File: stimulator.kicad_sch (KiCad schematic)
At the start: 1 part, among them U1 ENS001-A2

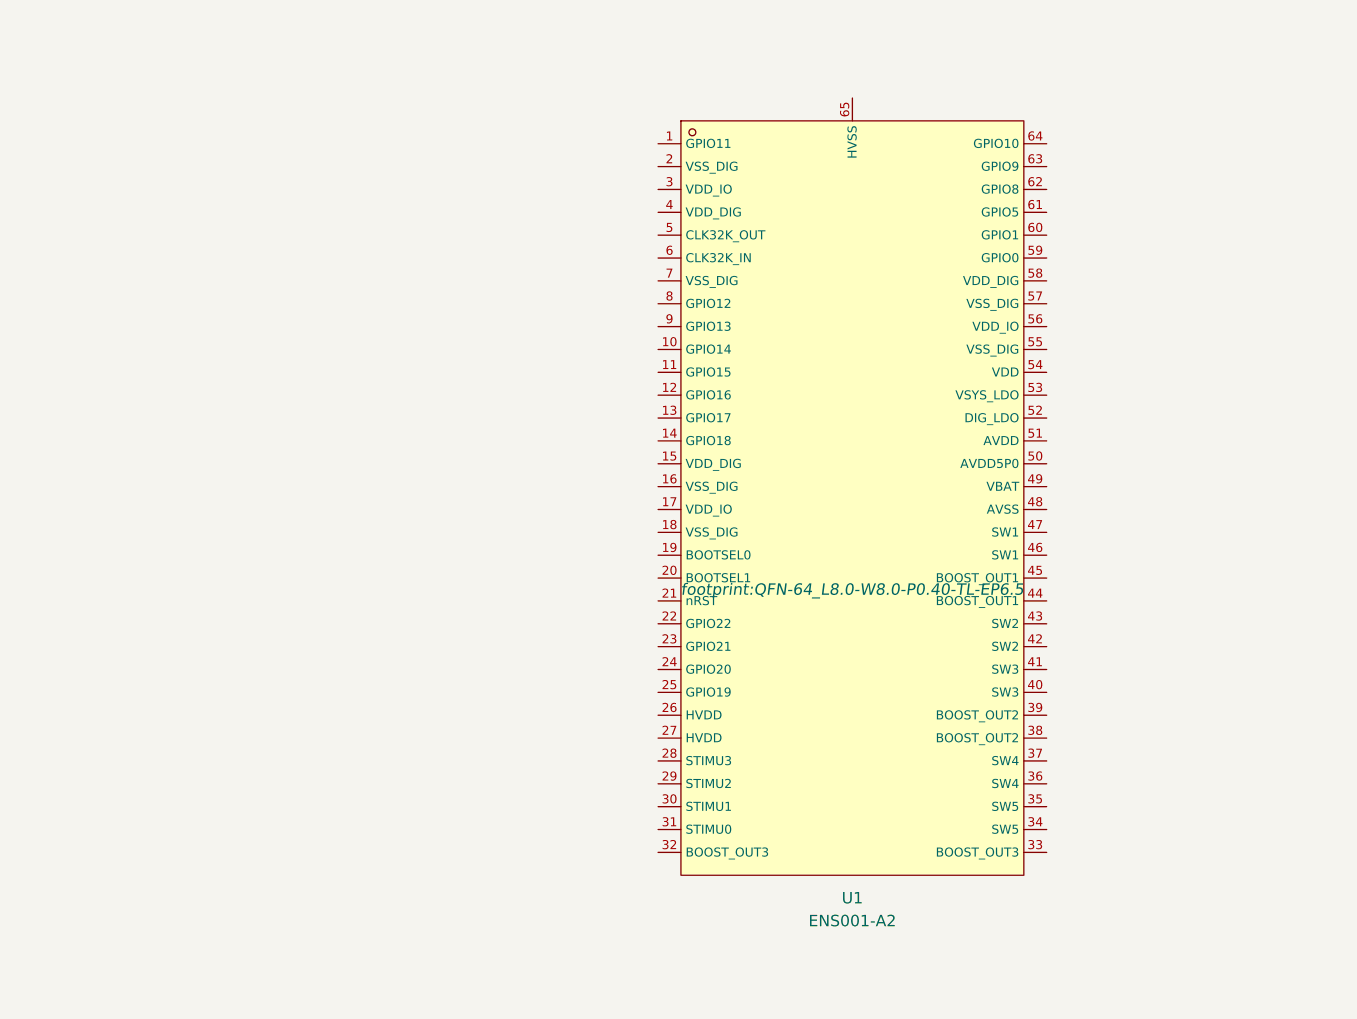
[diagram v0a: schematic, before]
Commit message: pin names assigned
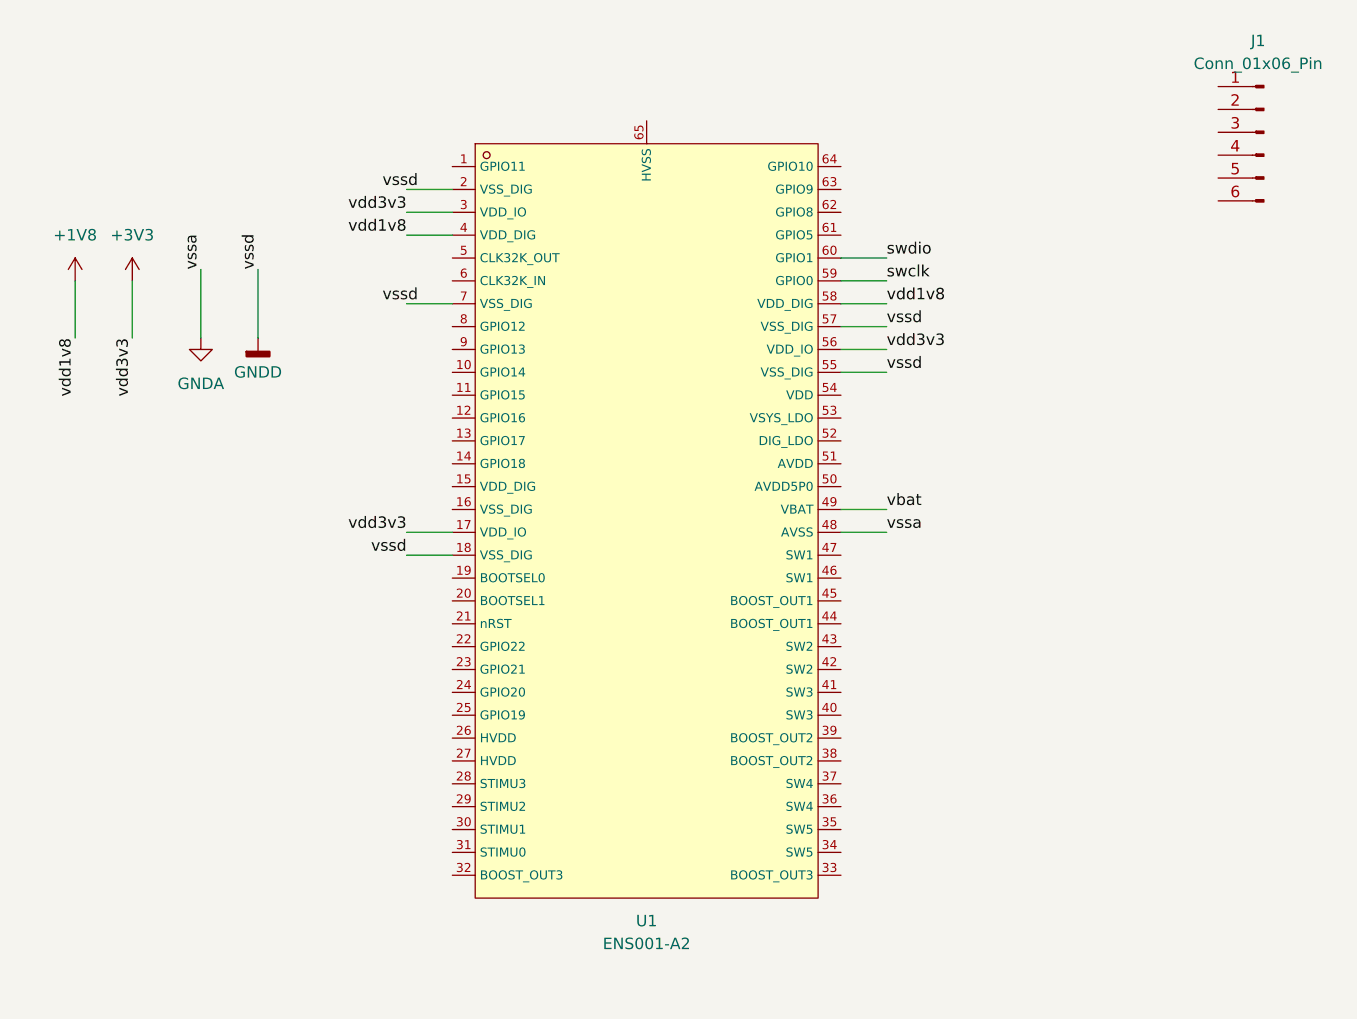
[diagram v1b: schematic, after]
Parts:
- added J1: Conn_01x06_Pin, symbol Connector:Conn_01x06_Pin
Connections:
- net +3V3: now reaches U1.17 (VDD_IO)
- net +3V3: now also U1.3 (VDD_IO), U1.56 (VDD_IO)
- net GNDD: now reaches U1.18 (VSS_DIG)
- net GNDD: now also U1.2 (VSS_DIG), U1.55 (VSS_DIG), U1.57 (VSS_DIG), U1.7 (VSS_DIG)
- net +1V8: now reaches U1.4 (VDD_DIG)
- net +1V8: now also U1.58 (VDD_DIG)
- net GNDA: now reaches U1.48 (AVSS)
- net vbat: now reaches U1.49 (VBAT)
- net swclk: now reaches U1.59 (GPIO0)
- net swdio: now reaches U1.60 (GPIO1)
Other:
- moved on the sheet: U1

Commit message: esp connected
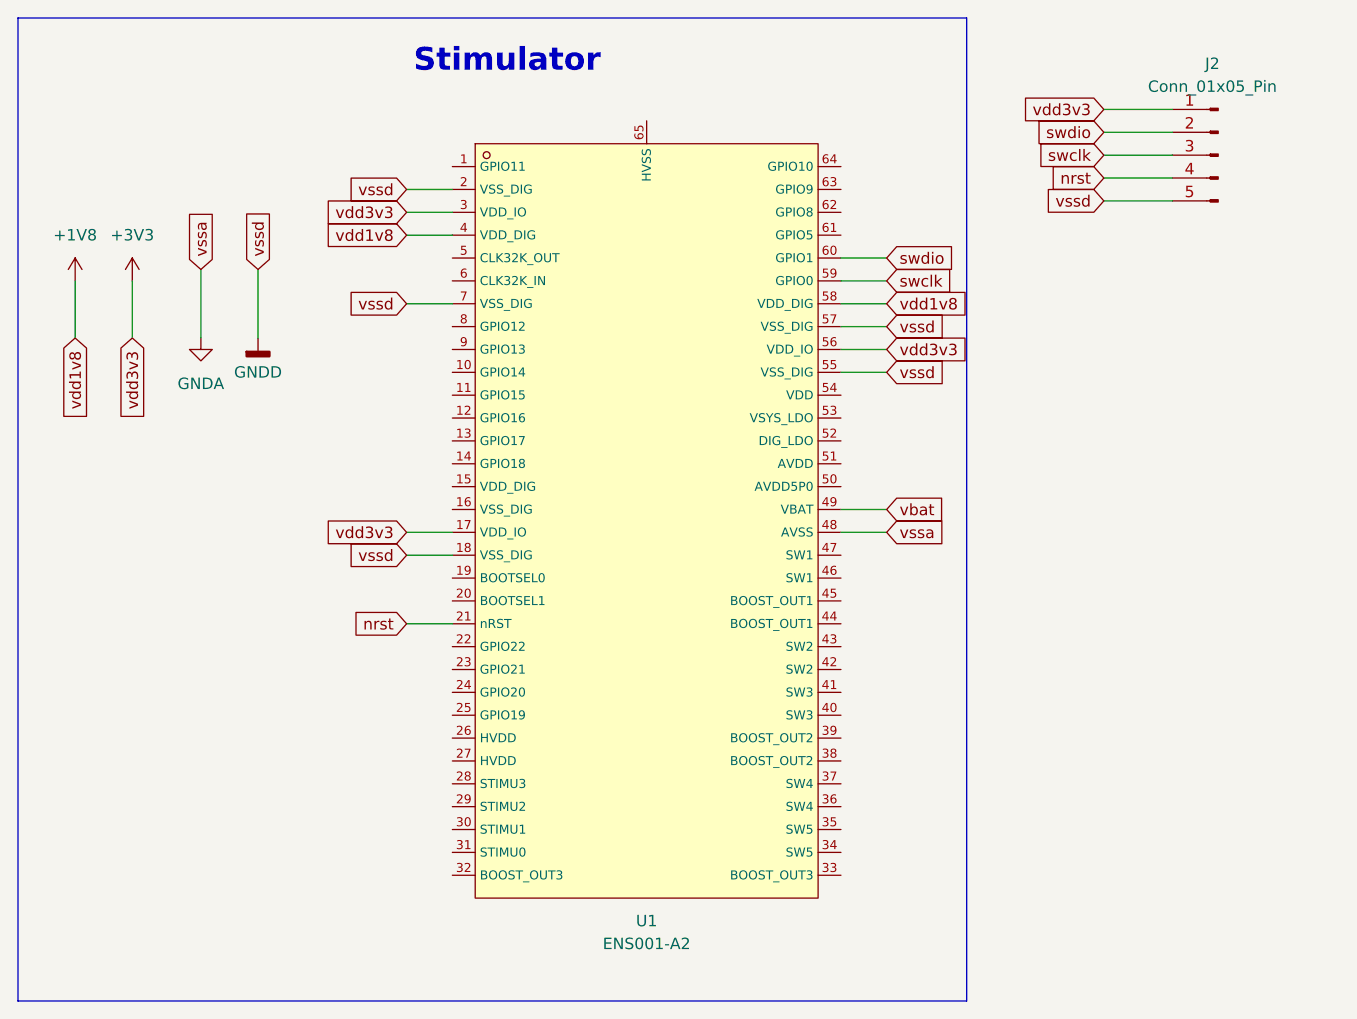
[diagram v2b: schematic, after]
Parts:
- removed J1: Conn_01x06_Pin, symbol Connector:Conn_01x06_Pin
- added J2: Conn_01x05_Pin, Connector_JST:JST_EH_B5B-EH-A_1x05_P2.50mm_Vertical, symbol Connector:Conn_01x05_Pin
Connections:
- net +3V3: now also J2.1 (Pin_1)
- net GNDD: now also J2.5 (Pin_5)
- net swclk: now also J2.3 (Pin_3)
- net swdio: now also J2.2 (Pin_2)
- net nrst: now reaches U1.21 (nRST)
- net nrst: now also J2.4 (Pin_4)
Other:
- note added: "Stimulator"
